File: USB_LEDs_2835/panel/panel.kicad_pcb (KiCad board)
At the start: 2 copper layers, 99.9 x 100 mm, 280 parts, among them U1 MT9284_1, U2 JL8022W-L, U3 74LVC1G04

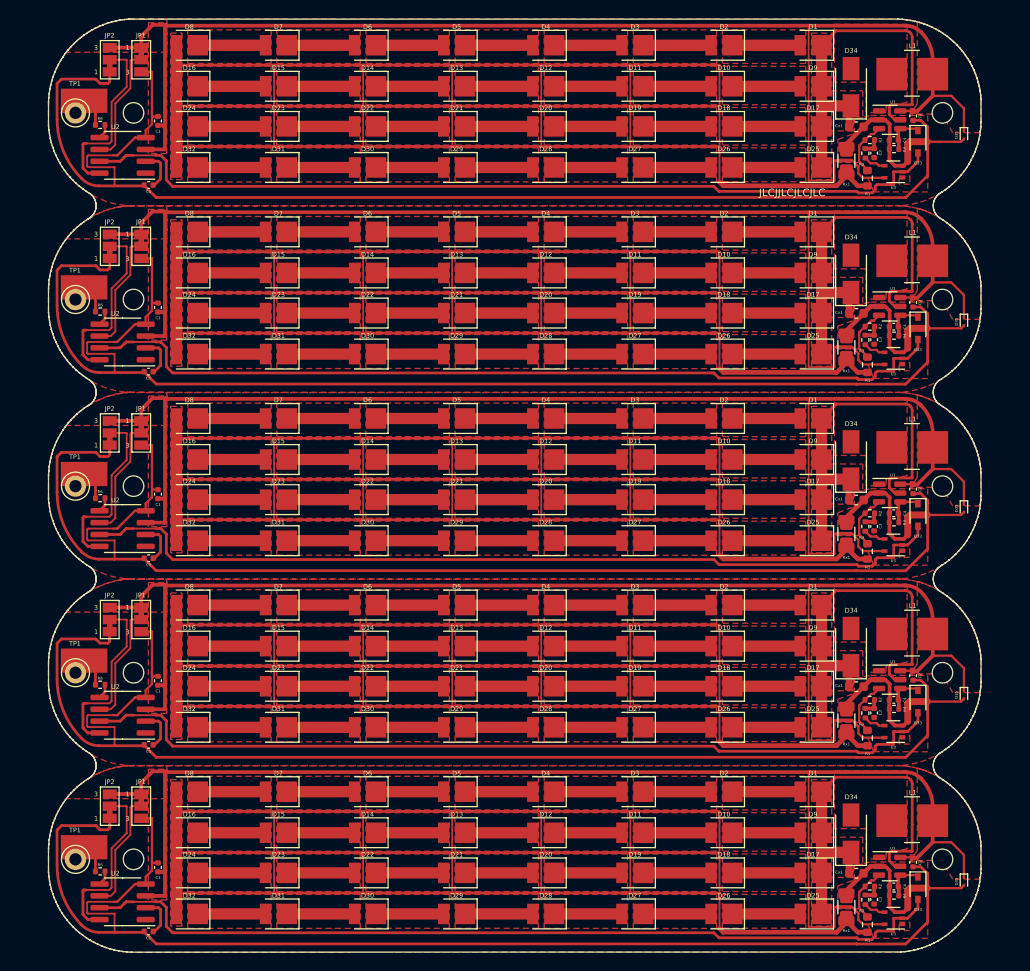
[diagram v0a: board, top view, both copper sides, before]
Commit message: Add files via upload
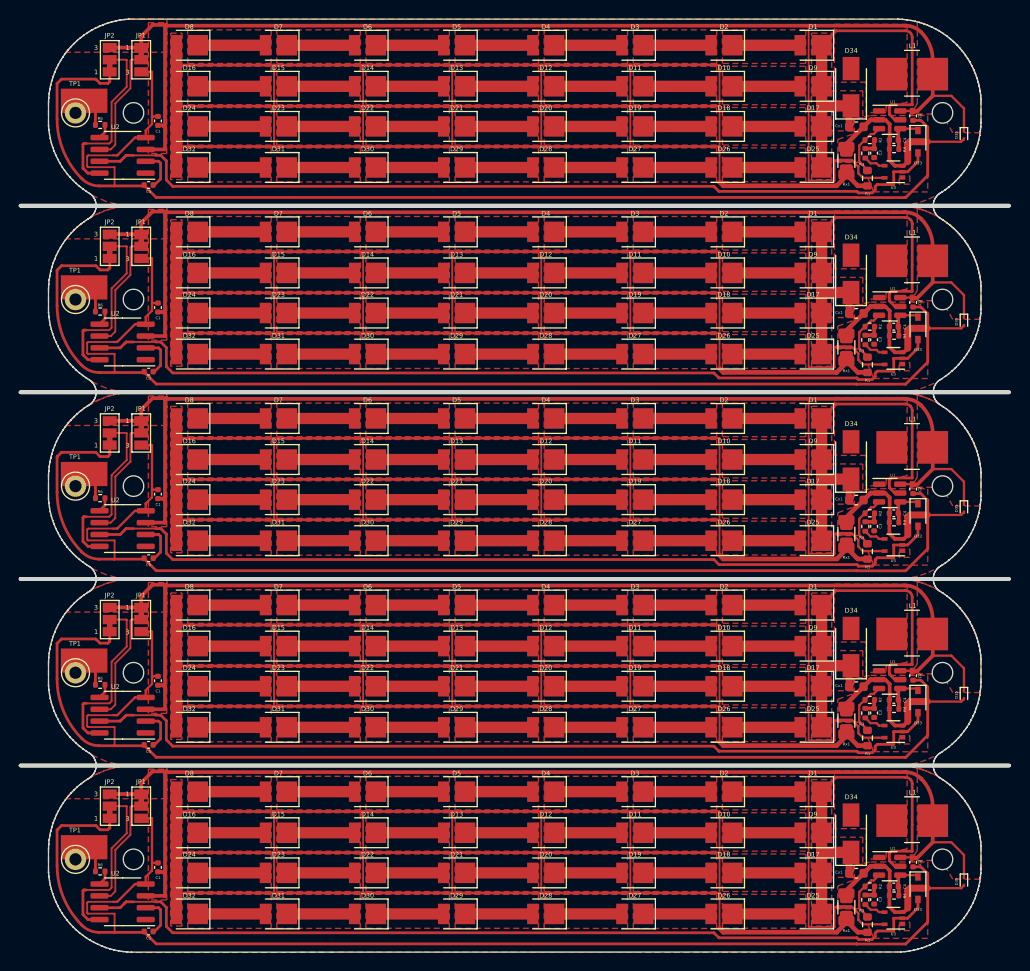
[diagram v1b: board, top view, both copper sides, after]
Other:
- board size 99.9 x 100 mm -> 105.9 x 100 mm
- board text added: "V-CUT"
- board text removed: "JLCJJLCJLCJLC"
- board text removed: "V Cut"
